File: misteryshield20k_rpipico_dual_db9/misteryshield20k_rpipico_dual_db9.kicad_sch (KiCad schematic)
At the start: 55 parts, among them J1 Joystick, J2 Joystick, J4 Conn_01x20_Pin, J5 Conn_01x02_Pin, J7 Conn_01x20_Pin, Q1 2N7002, Q10 2N7002, Q11 2N7002, Q12 2N7002, Q2 2N7002, Q3 2N7002, Q4 2N7002, Q5 2N7002, Q6 2N7002, Q7 2N7002, Q8 2N7002, Q9 2N7002, U1 USB_C_Receptacle_PowerOnly_6P

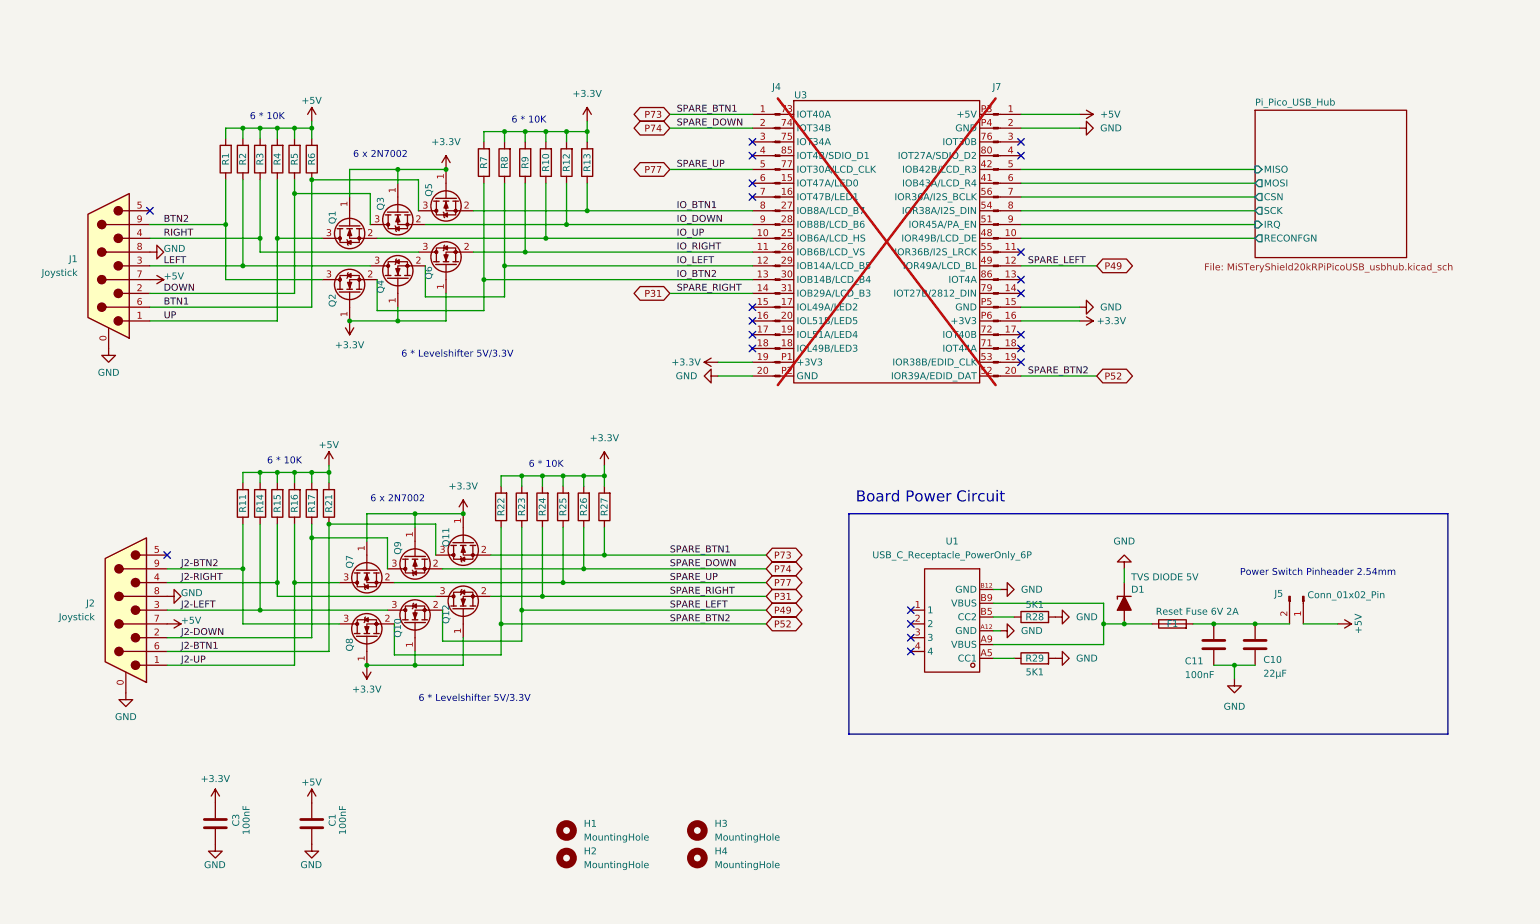
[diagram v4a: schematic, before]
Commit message: Add files via upload
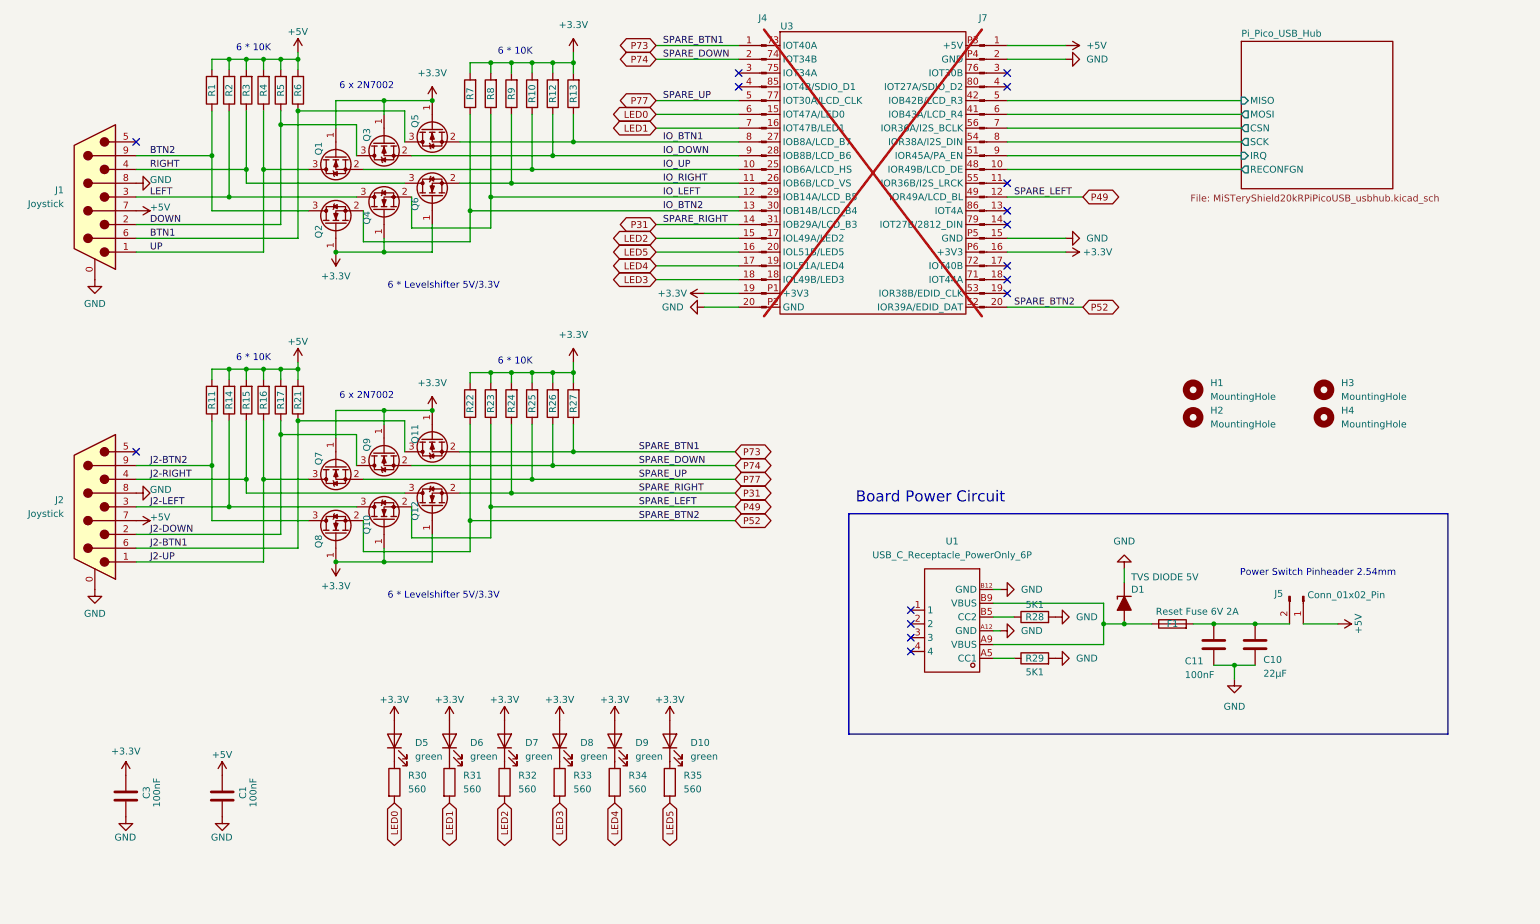
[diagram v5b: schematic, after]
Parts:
- added D10, D5, D6, D7, D8, D9: green, LED_SMD:LED_0805_2012Metric, symbol Device:LED
- added R30, R31, R32, R33, R34, R35: 560, Resistor_SMD:R_0805_2012Metric, symbol Device:R
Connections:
- net +3.3V: now also D10.2 (A), D5.2 (A), D6.2 (A), D7.2 (A), D8.2 (A), D9.2 (A)
- net LED2: now reaches J4.15 (Pin_15)
- net LED2: now also R32.2
- net LED5: now reaches J4.16 (Pin_16)
- net LED5: now also R35.2
- net LED4: now reaches J4.17 (Pin_17)
- net LED4: now also R34.2
- net LED3: now reaches J4.18 (Pin_18)
- net LED3: now also R33.2
- net LED0: now reaches J4.6 (Pin_6)
- net LED0: now also R30.2
- net LED1: now reaches J4.7 (Pin_7)
- net LED1: now also R31.2
- new net: D8.1 (K), R33.1
- new net: D9.1 (K), R34.1
- new net: D5.1 (K), R30.1
- new net: D6.1 (K), R31.1
- new net: D7.1 (K), R32.1
- new net: D10.1 (K), R35.1
- no-connect marks 22 -> 16
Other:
- moved on the sheet: C1, C3, H1, H2, H3, H4, J1, J2, J4, J7, Q1, Q10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

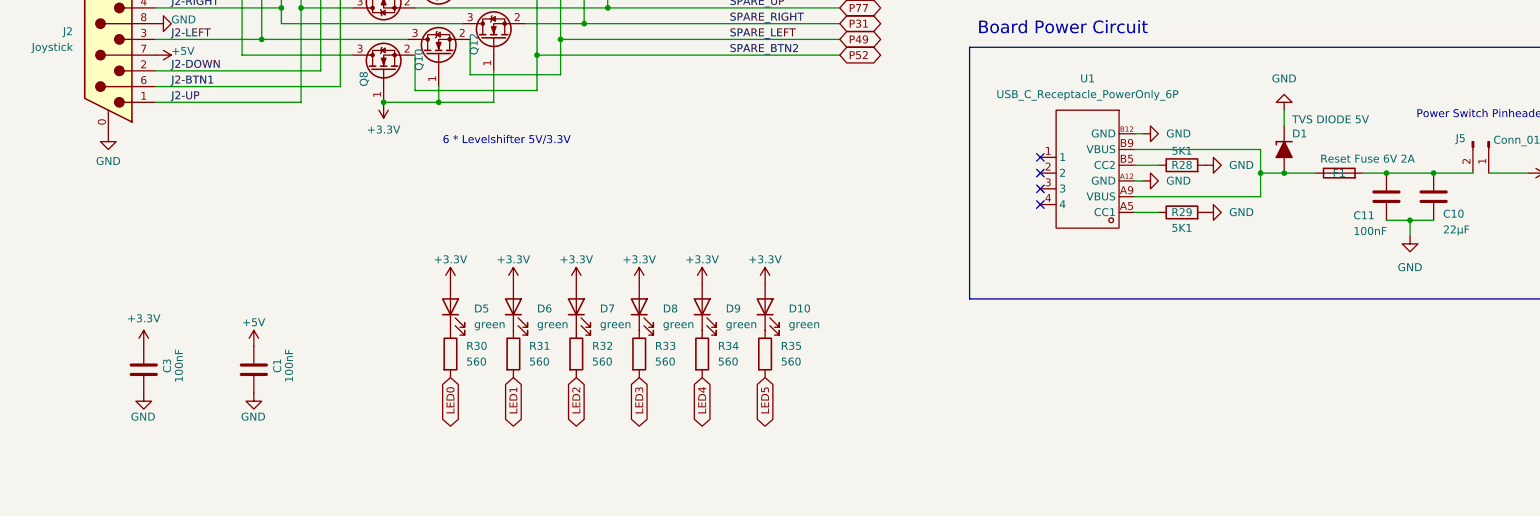
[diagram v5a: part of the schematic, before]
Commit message: Add files via upload
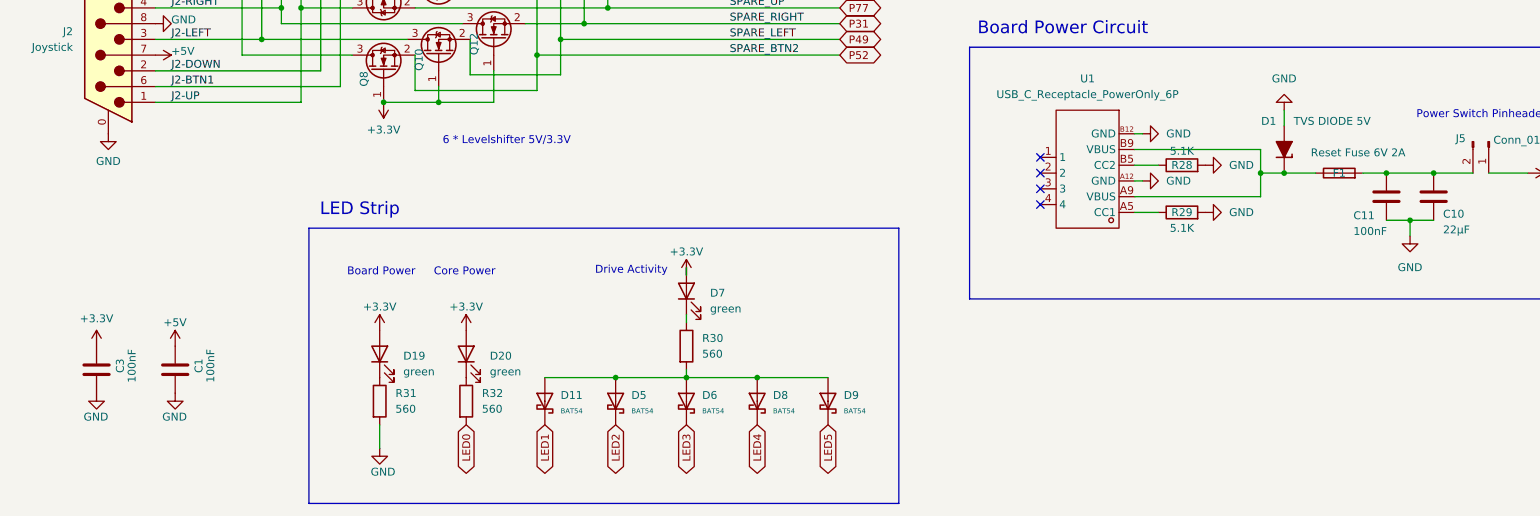
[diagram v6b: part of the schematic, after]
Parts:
- removed D10, D5, D6, D8, D9: green, LED_SMD:LED_0805_2012Metric, symbol Device:LED
- removed R33, R34, R35: 560, Resistor_SMD:R_0805_2012Metric, symbol Device:R
- added D11, D5, D6, D8, D9: BAT54, PCM_JLCPCB:D_SOT-23, symbol PCM_JLCPCB-Diodes:Schottky,BAT54
- added D19, D20: green, LED_SMD:LED_0805_2012Metric, symbol Device:LED
- R28, R29: value 5K1 -> 5.1K
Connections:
- net +3.3V: now also D19.2 (A), D20.2 (A)
- net GND: now also D1.2 (A), R31.2; no longer D1.1 (K)
- net LED0: now also R32.2; no longer R30.2
- net LED1: now also D11.3; no longer R31.2
- net LED2: now also D5.3; no longer R32.2
- net LED3: now also D6.3
- net LED4: now also D8.3
- net LED5: now also D9.3
- net at F1.1, U1.A9 (VBUS), U1.B9 (VBUS): now also D1.1 (K); no longer D1.2 (A)
- net at R30.1: now also D7.1 (K)
- net at R31.1: now also D19.1 (K)
- net at R32.1: now also D20.1 (K); no longer D7.1 (K)
- new net: D11.1, D5.1, D6.1, D8.1, D9.1, R30.2
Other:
- note added: "Board Power"
- note added: "Core Power"
- note added: "Drive Activity"
- note added: "LED Strip"
- moved on the sheet: C1, C3, D1
